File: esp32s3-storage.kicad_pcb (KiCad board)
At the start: 2 copper layers, 56.9 x 40.4 mm, 32 parts, among them J1 USB_C_Receptacle_USB2.0_14P, J2 Conn_01x02, J3 Micro_SD_Card, J4 Conn_01x08_Socket, J5 Conn_01x15_Pin, Q1 CJ3401, SW1 SW_Push, SW2 SW_Push, SW3 SW_Push, SW4 SW_Push, U1 ESP32-S3-WROOM-1, U2 AMS1117-3.3

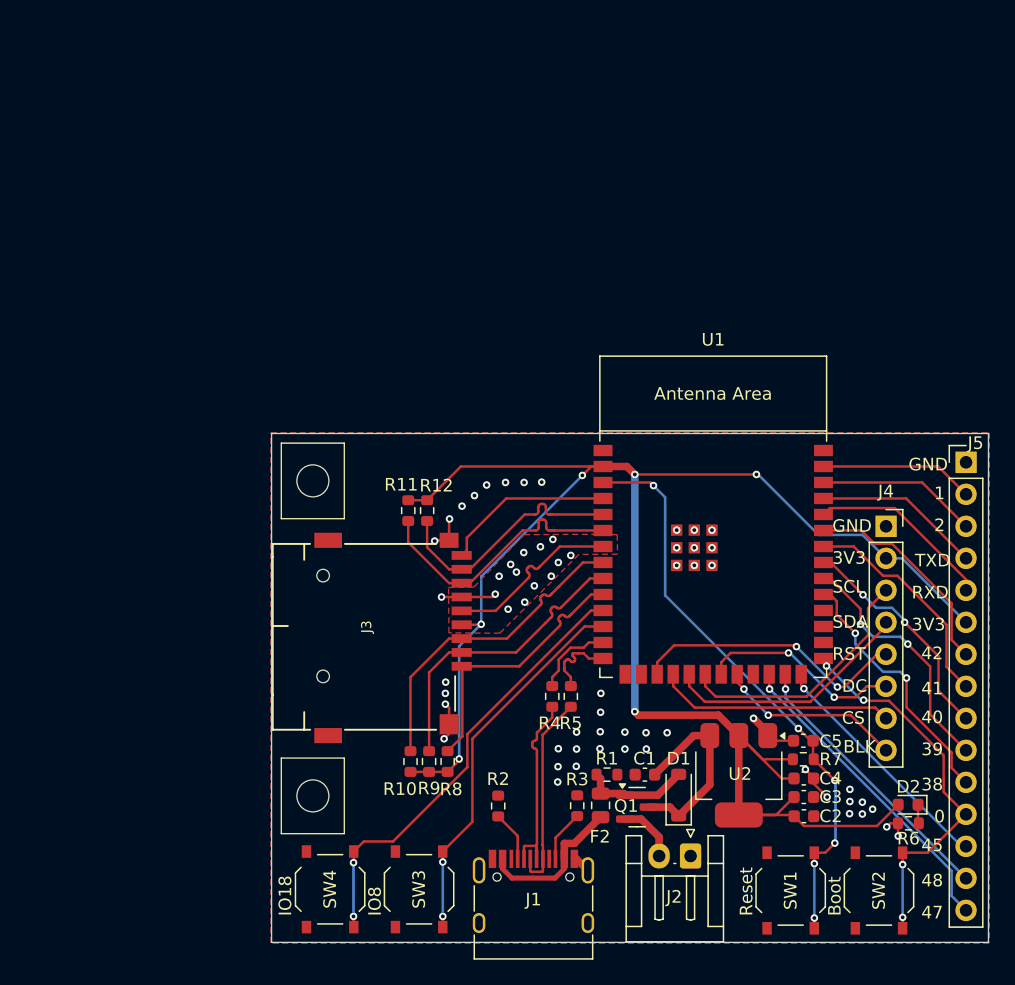
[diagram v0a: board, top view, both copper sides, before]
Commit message: esp32s3-storage v3
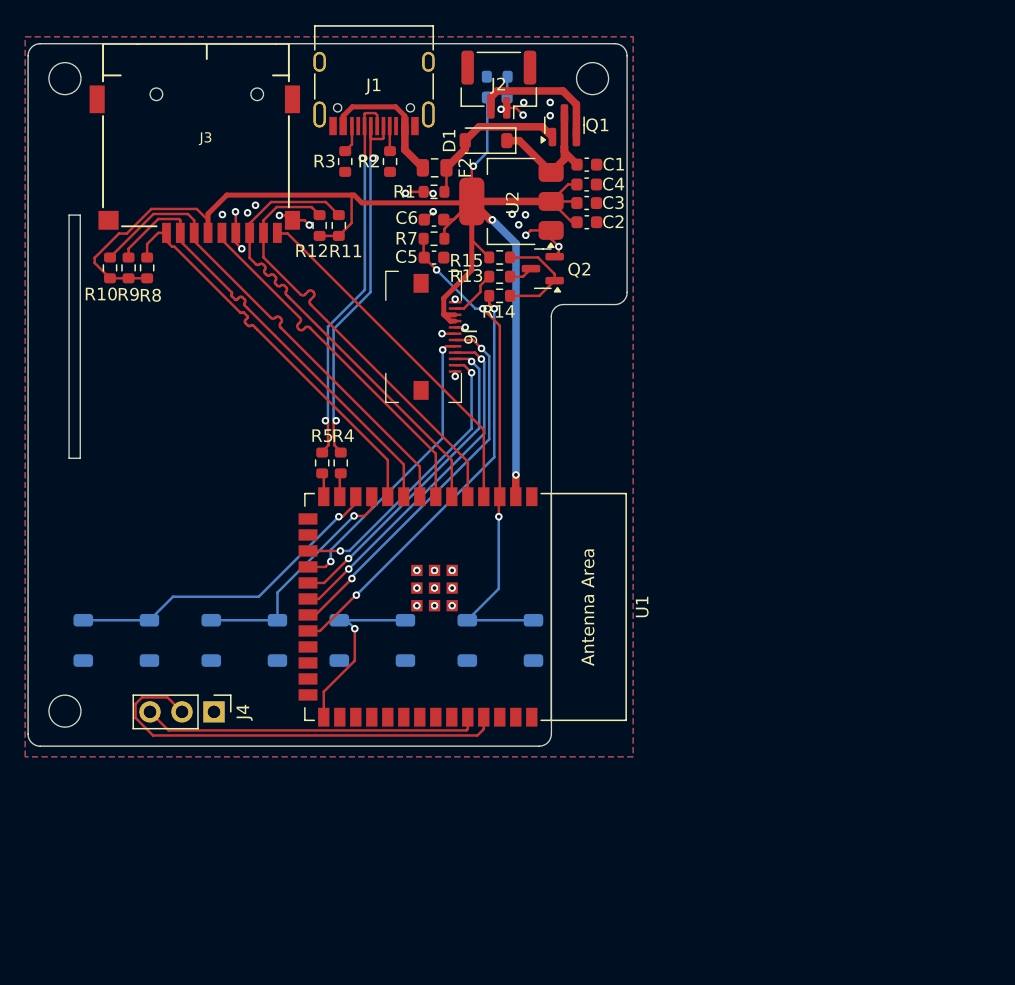
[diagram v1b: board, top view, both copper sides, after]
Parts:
- removed J5: Conn_01x15_Pin, Connector_PinHeader_2.54mm:PinHeader_1x15_P2.54mm_Vertical
- added C6: 0.1uF, Capacitor_SMD:C_0603_1608Metric, F.Cu at (148.5, 80.6)
- added J6: ~, user_created:fpc connector 1x12 P0.5mm bottom-side back-flip, F.Cu at (148.8, 89.9)
- added Q2: SS8050, Package_TO_SOT_SMD:SOT-23, F.Cu at (157.2, 84.5)
- added R13: 10R, Resistor_SMD:R_0603_1608Metric, F.Cu at (153.7, 85.1)
- added R14: 1K, Resistor_SMD:R_0603_1608Metric, F.Cu at (153.7, 86.6)
- added R15: 10K, Resistor_SMD:R_0603_1608Metric, F.Cu at (153.7, 83.6)
- D2, R6: moved to B.Cu
- J2: footprint Connector_JST:JST_EH_S2B-EH_1x02_P2.50mm_Horizontal -> Connector_JST:JST_GH_SM02B-GHS-TB_1x02-1MP_P1.25mm_Horizontal
- J4: value Conn_01x08_Socket -> Conn_01x03_Pin; footprint Connector_PinSocket_2.54mm:PinSocket_1x08_P2.54mm_Vertical -> Connector_PinHeader_2.54mm:PinHeader_1x03_P2.54mm_Vertical
- SW1, SW2, SW3, SW4: footprint Button_Switch_SMD:SW_Push_1P1T_XKB_TS-1187A -> Button_Switch_SMD:SW_SPST_PTS647_Sx38; moved to B.Cu
- moved R6 67.7 mm to (153.5, 69.2)
- moved J1 67.5 mm to (143.8, 69.1), turned to 180 degrees
- moved D2 64.9 mm to (153.5, 70.9)
- moved J2 63.1 mm to (153.7, 69.8)
- moved J4 55.3 mm to (131.1, 119.6), turned to -90 degrees
- moved Q1 54.4 mm to (158.9, 73.1), turned to 90 degrees
- moved R3 54.3 mm to (141.5, 75.9), turned to -90 degrees
- moved D1 54.2 mm to (152.7, 74.3), turned to 180 degrees
- moved F2 52.3 mm to (148.6, 76.5), turned to 0 degrees
- moved R2 51.9 mm to (145.0, 75.9), turned to -90 degrees
- moved R7 50.7 mm to (148.5, 82.1), turned to 180 degrees
- moved C2 50.2 mm to (160.7, 80.8)
- moved C3 50.2 mm to (160.6, 79.2)
- moved C4 50.2 mm to (160.6, 77.8)
- moved U2 49.0 mm to (154.7, 79.1), turned to 180 degrees
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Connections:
- J4 pad 2: /3V3 -> /TXD0
- J4 pad 3: /LCD_SCL -> /RXD0
- U1 pad 15: unconnected-(U1-IO3-Pad15) -> /GPIO3_S
- U1 pad 16: unconnected-(U1-IO46-Pad16) -> /GPIO46_S
- U1 pad 23: unconnected-(U1-IO21-Pad23) -> /GPIO21
- U1 pad 26: /GPIO45 -> /GPIO45_S
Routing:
- net /3V3: track 148.6 -> 116.9 mm, vias 6 -> 3
- net /GPIO47: track 25.2 -> 0.00 mm, vias 1 -> 0
- net /GPIO48: track 22.1 -> 0.00 mm, vias 1 -> 0
- net /TXD0: track 13.3 -> 34.9 mm
- net /GPIO38: track 20.7 -> 0.00 mm, vias 2 -> 0
- net /GPIO39: track 19.9 -> 0.00 mm, vias 2 -> 0
- net /GPIO45: track 19.3 -> 0.00 mm, vias 1 -> 0
- net /LCD_BLK: track 14.8 -> 33.5 mm
- net /GPIO40: track 18.1 -> 0.00 mm, vias 2 -> 0
- net /GPIO41: track 17.9 -> 0.00 mm
- net /GPIO42: track 17.1 -> 0.00 mm
- net /GPIO18: track 35.3 -> 18.6 mm, vias 2 -> 1
- net /SDHOST_DAT0: track 21.5 -> 37.8 mm
- net /BOOT: track 30.6 -> 15.1 mm, vias 4 -> 1
- net /SDHOST_DAT1: track 19.8 -> 35.1 mm
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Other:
- board size 56.9 x 40.4 mm -> 47.6 x 55.8 mm
- board text removed: "0"
- board text removed: "1"
- board text removed: "2"
- board text removed: "38"
- board text removed: "39"
- board text removed: "3V3"
- board text removed: "40"
- board text removed: "41"
- board text removed: "42"
- board text removed: "45"
- board text removed: "47"
- board text removed: "48"
- board text removed: "BLK"
- board text removed: "Boot"
- board text removed: "CS"
- board text removed: "DC"
- board text removed: "GND"
- board text removed: "IO18"
- board text removed: "IO8"
- board text removed: "RST"
- board text removed: "RXD"
- board text removed: "Reset"
- board text removed: "SCL"
- board text removed: "SDA"
- board text removed: "TXD"
